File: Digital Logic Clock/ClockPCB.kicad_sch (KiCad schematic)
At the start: 12 parts, among them J1 Barrel_Jack, U1 4081

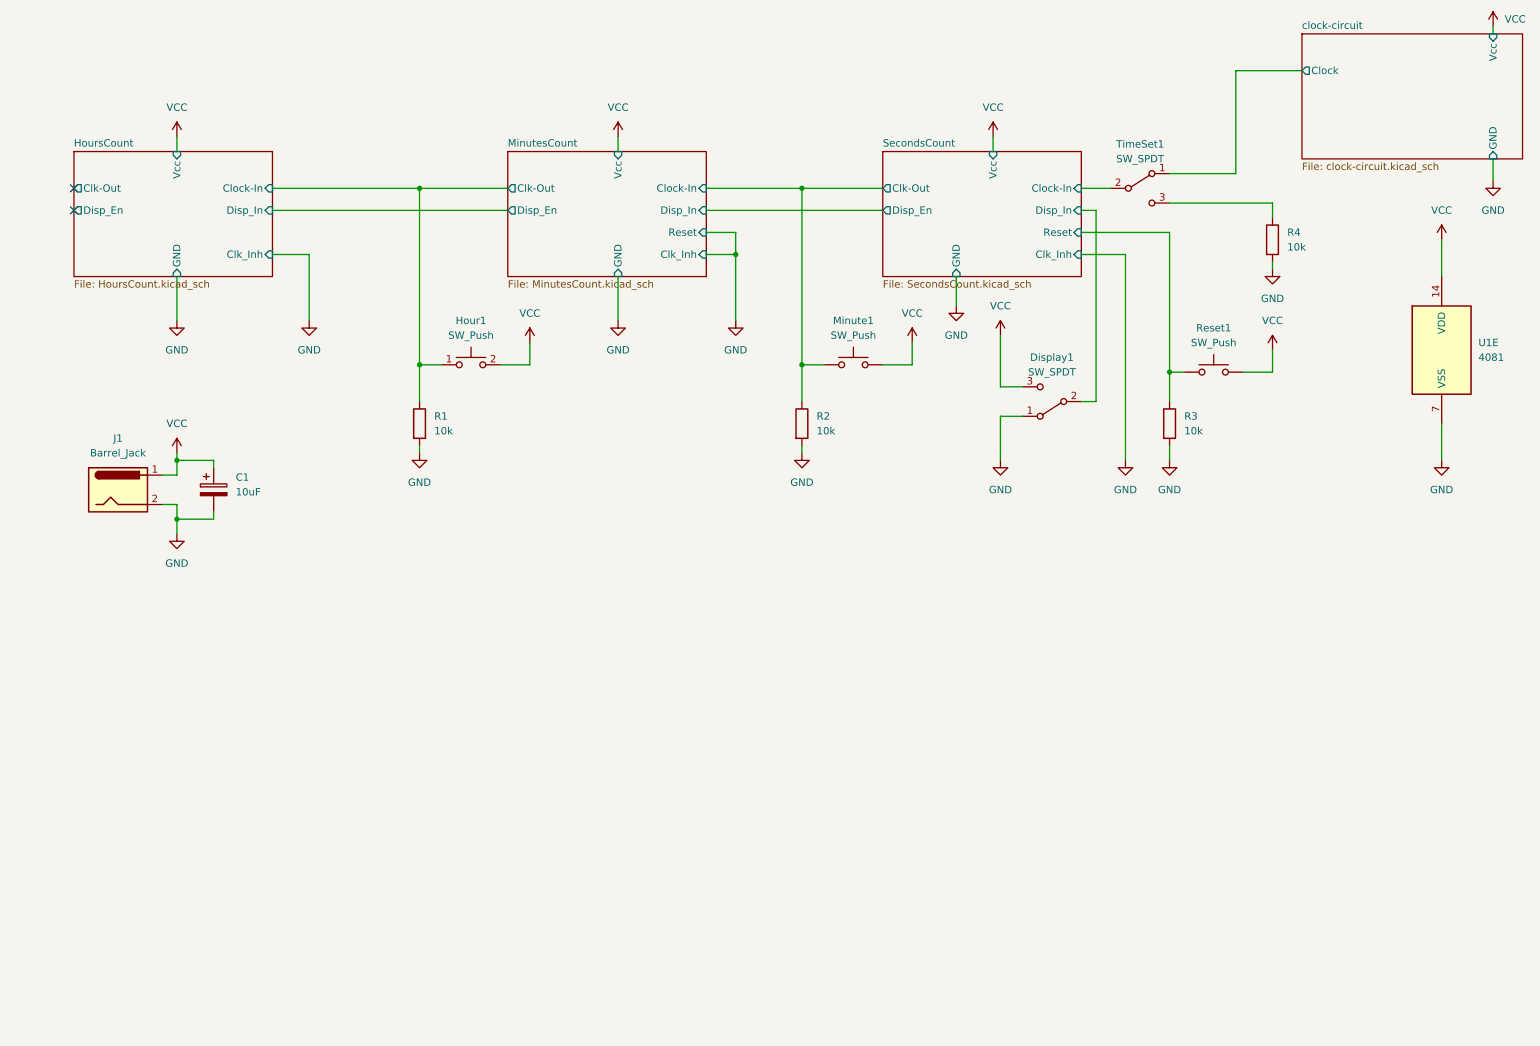
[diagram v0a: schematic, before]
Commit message: Clock Project
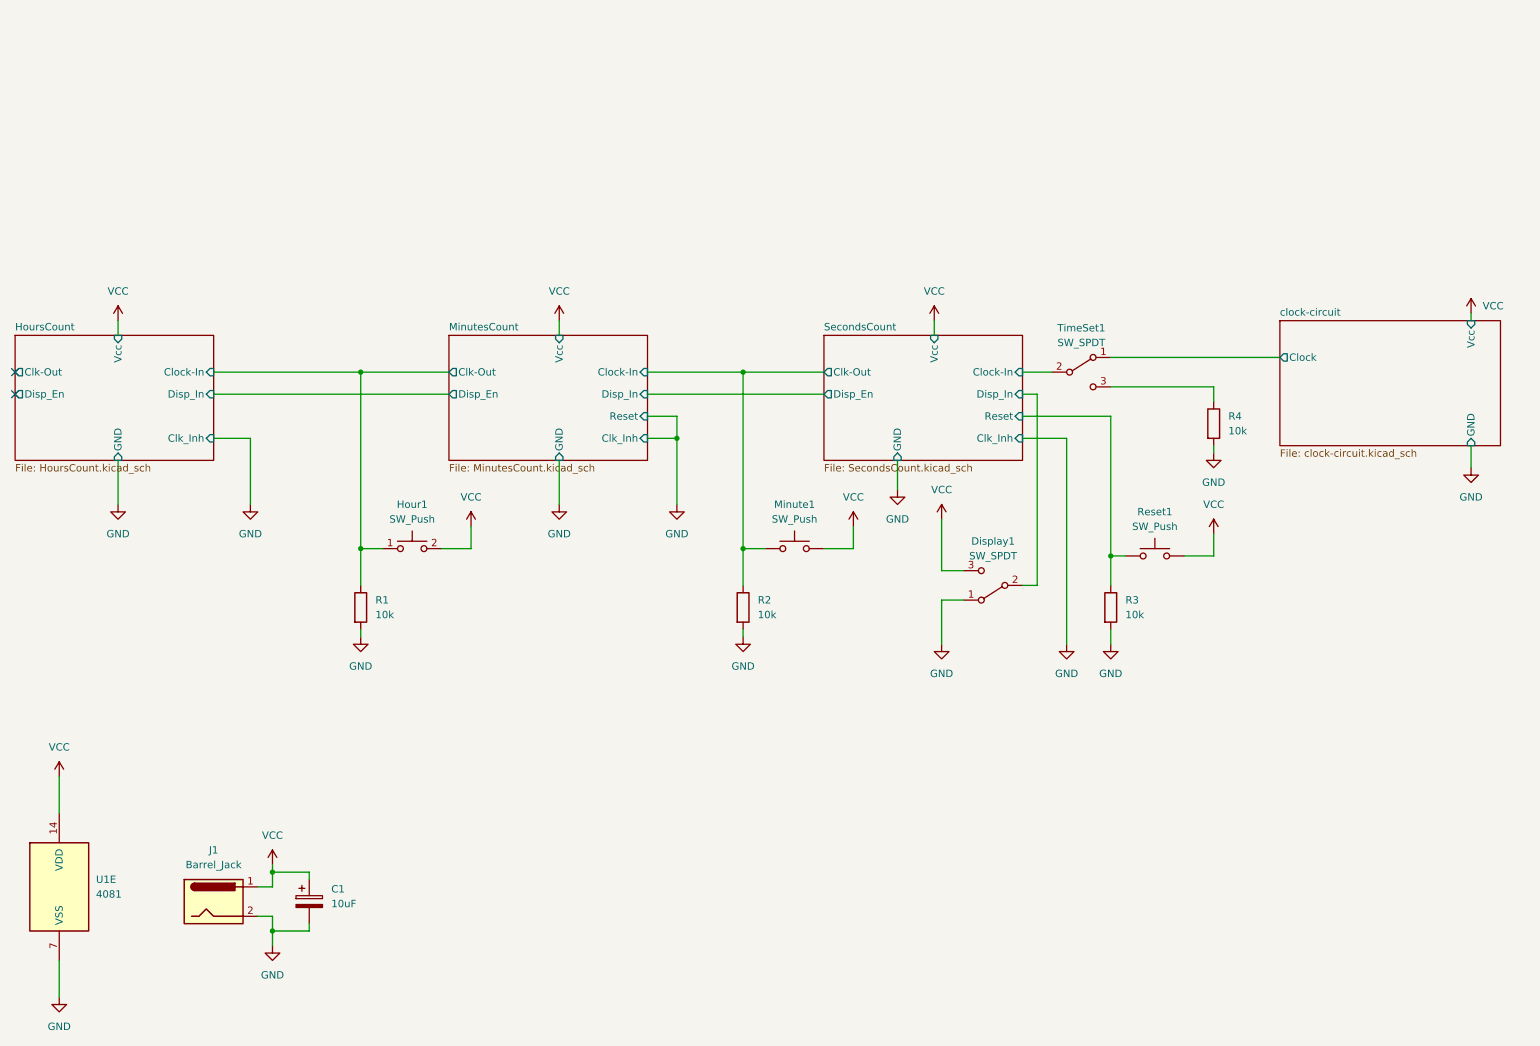
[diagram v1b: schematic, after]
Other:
- company: (none) -> Akbar Q
- title: (none) -> Practise Project to Test JLC PCB
- moved on the sheet: C1, Display1, Hour1, J1, Minute1, R1, R2, R3, R4, Reset1, TimeSet1, U1E
